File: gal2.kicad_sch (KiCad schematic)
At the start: 1 part, among them IC1 D65101GD055

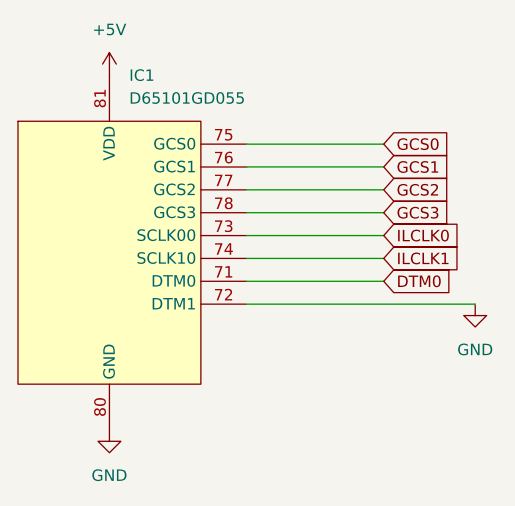
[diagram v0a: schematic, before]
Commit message: wire power lines
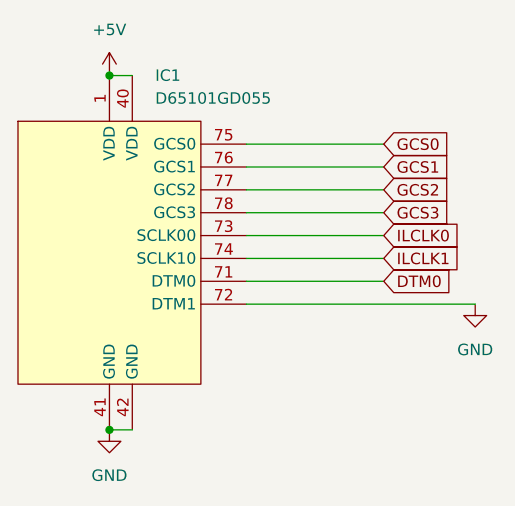
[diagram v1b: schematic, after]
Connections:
- net +5V: now also IC1.1 (VDD), IC1.40 (VDD); no longer IC1.81 (VDD)
- net GND: now also IC1.41 (GND), IC1.42 (GND); no longer IC1.80 (GND)
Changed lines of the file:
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@@
 (kicad_sch (version 20230121) (generator eeschema)
   (paper "A4")
+  (junction (at 48.26 127) (diameter 0) (color 0 0 0 0)
+  )
+  (junction (at 48.26 166.37) (diameter 0) (color 0 0 0 0)
+  )
   (wire (pts (xy 63.5 139.7) (xy 78.74 139.7))
     (stroke (width 0) (type default))
   )
   (wire (pts (xy 63.5 147.32) (xy 78.74 147.32))
+    (stroke (width 0) (type default))
+  )
+  (wire (pts (xy 48.26 127) (xy 50.8 127))
     (stroke (width 0) (type default))
   )
@@
   )
   (wire (pts (xy 63.5 142.24) (xy 78.74 142.24))
+    (stroke (width 0) (type default))
+  )
+  (wire (pts (xy 48.26 166.37) (xy 50.8 166.37))
     (stroke (width 0) (type default))
   )
@@
   (symbol (lib_id "88va_Library:GAL") (at 48.26 132.08 0) (unit 1)
     (in_bom yes) (on_board yes) (dnp no) (fields_autoplaced)
-    (property "Reference" "IC1" (at 50.4541 127 0)
+    (property "Reference" "IC1" (at 53.34 127 0)
       (effects (font (size 1.27 1.27)) (justify left))
     )
-    (property "Value" "D65101GD055\n" (at 50.4541 129.54 0)
+    (property "Value" "D65101GD055\n" (at 53.34 129.54 0)
       (effects (font (size 1.27 1.27)) (justify left))
     )
@@
       (effects (font (size 1.27 1.27)) hide)
     )
-    (pin "80")
+    (pin "1")
     (pin "75")
     (pin "76")
-    (pin "81")
+    (pin "41")
     (pin "77")
     (pin "71")
@@
     (pin "78")
     (pin "72")
+    (pin "42")
+    (pin "40")
     (instances
       (project "88va2-circuit"
